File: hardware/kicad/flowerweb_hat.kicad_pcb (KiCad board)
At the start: 2 copper layers, 65 x 56.5 mm, 18 parts, among them J1 PJ-063AH, J2 PJ-063AH, J3 Raspberry Pi 40-pin, J4 STATUS LED, Q1 TIP121, U1 MT3608 module

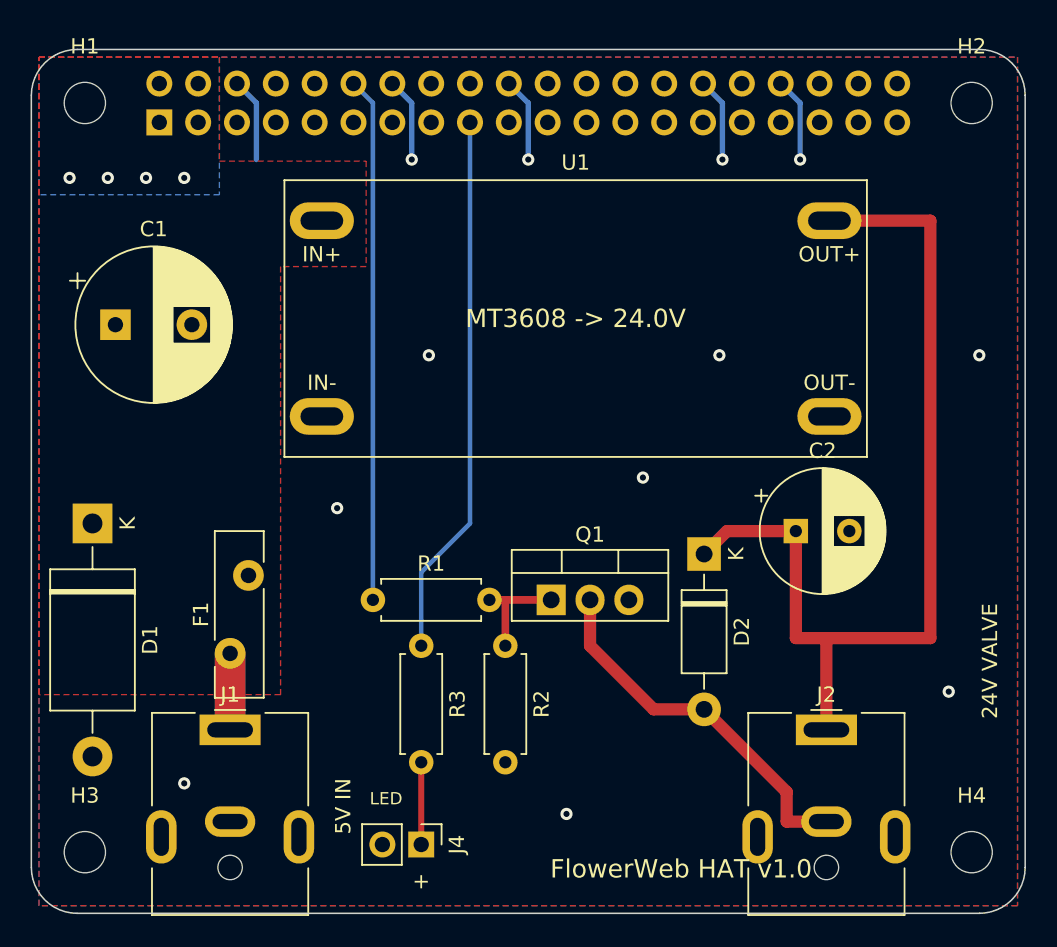
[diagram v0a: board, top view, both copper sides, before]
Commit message: bug fixes
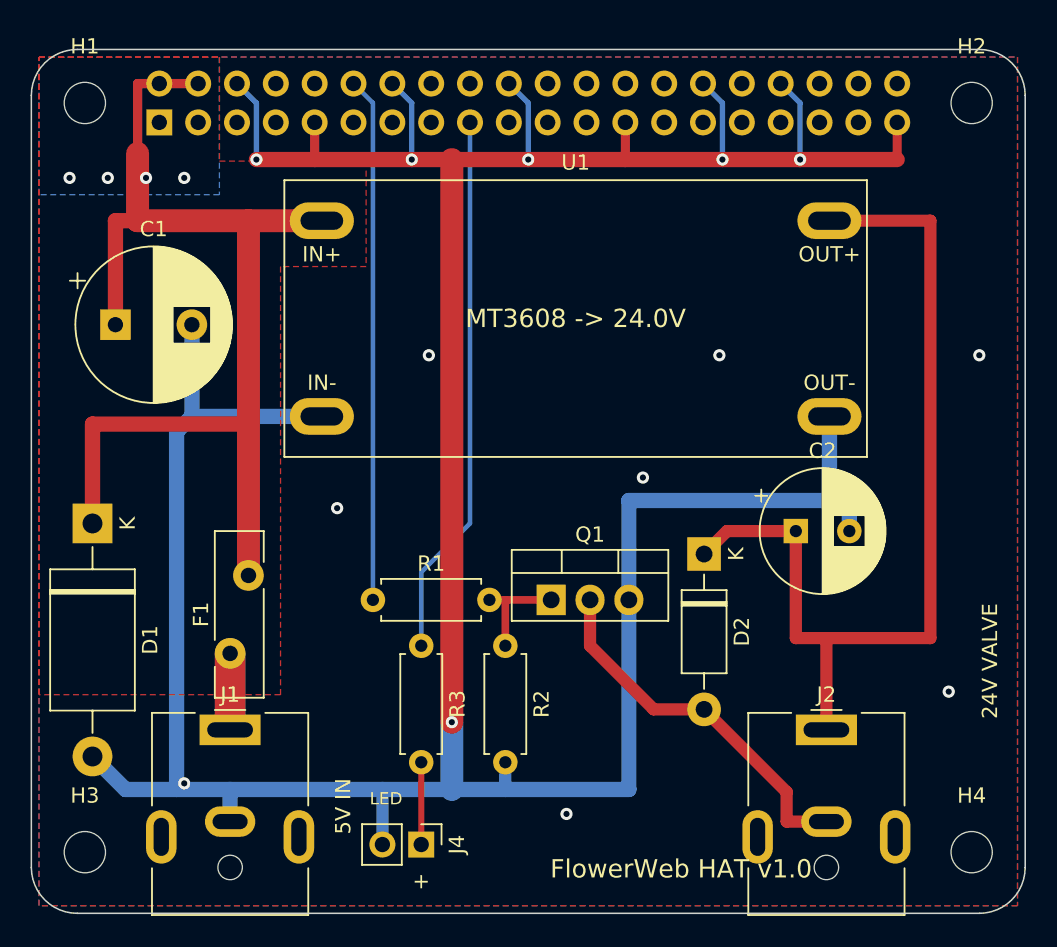
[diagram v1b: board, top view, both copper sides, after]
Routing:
- net GND: track 27.5 -> 241.5 mm, vias 12 -> 14
- net +5V: track 0.00 -> 83.4 mm
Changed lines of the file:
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@@
   (segment (start 149.01 102.23) (end 150.28 103.5) (width 0.35) (layer "B.Cu") (net 1))
   (segment (start 150.28 103.5) (end 150.28 107.2) (width 0.35) (layer "B.Cu") (net 1))
+  (segment (start 114.2 134.4) (end 114.2 111.2) (width 1.5) (layer "F.Cu") (net 2))
+  (segment (start 114.2 111.2) (end 119 111.2) (width 1.5) (layer "F.Cu") (net 2))
+  (segment (start 114.2 111.2) (end 106.95 111.2) (width 1.5) (layer "F.Cu") (net 2))
+  (segment (start 106.95 111.2) (end 106.95 106.8) (width 1.5) (layer "F.Cu") (net 2))
+  (segment (start 106.95 106.8) (end 106.95 102.23) (width 0.6) (layer "F.Cu") (net 2))
+  (segment (start 106.95 102.23) (end 108.37 102.23) (width 0.6) (layer "F.Cu") (net 2))
+  (segment (start 108.37 102.23) (end 110.91 102.23) (width 0.6) (layer "F.Cu") (net 2))
+  (segment (start 107.5 108.4) (end 106.95 106.8) (width 0.6) (layer "B.Cu") (net 2))
+  (segment (start 106.95 106.8) (end 106.95 102.23) (width 0.6) (layer "B.Cu") (net 2))
+  (segment (start 106.95 102.23) (end 108.37 102.23) (width 0.6) (layer "B.Cu") (net 2))
+  (segment (start 108.37 102.23) (end 110.91 102.23) (width 0.6) (layer "B.Cu") (net 2))
+  (segment (start 105.5 118) (end 105.5 111.2) (width 1) (layer "F.Cu") (net 2))
+  (segment (start 105.5 111.2) (end 106.95 111.2) (width 1) (layer "F.Cu") (net 2))
+  (segment (start 104 131) (end 104 124.5) (width 1) (layer "F.Cu") (net 2))
+  (segment (start 104 124.5) (end 114.2 124.5) (width 1) (layer "F.Cu") (net 2))
+  (segment (start 114.72 107.2) (end 118.53 107.2) (width 1) (layer "F.Cu") (net 1))
+  (segment (start 118.53 107.2) (end 124.88 107.2) (width 1) (layer "F.Cu") (net 1))
+  (segment (start 124.88 107.2) (end 127.5 107.2) (width 1) (layer "F.Cu") (net 1))
+  (segment (start 127.5 107.2) (end 132.5 107.2) (width 1) (layer "F.Cu") (net 1))
+  (segment (start 132.5 107.2) (end 138.85 107.2) (width 1) (layer "F.Cu") (net 1))
+  (segment (start 138.85 107.2) (end 145.2 107.2) (width 1) (layer "F.Cu") (net 1))
+  (segment (start 145.2 107.2) (end 150.28 107.2) (width 1) (layer "F.Cu") (net 1))
+  (segment (start 150.28 107.2) (end 156.63 107.2) (width 1) (layer "F.Cu") (net 1))
+  (segment (start 118.53 104.77) (end 118.53 107.2) (width 0.6) (layer "F.Cu") (net 1))
+  (segment (start 138.85 104.77) (end 138.85 107.2) (width 0.6) (layer "F.Cu") (net 1))
+  (segment (start 156.63 104.77) (end 156.63 107.2) (width 0.6) (layer "F.Cu") (net 1))
+  (segment (start 127.5 107.2) (end 127.5 144) (width 1.5) (layer "F.Cu") (net 1))
+  (segment (start 127.5 144) (end 127.5 148.4) (width 1.5) (layer "B.Cu") (net 1))
+  (segment (start 104 146.24) (end 106.16 148.4) (width 1) (layer "B.Cu") (net 1))
+  (segment (start 106.16 148.4) (end 109.5 148.4) (width 1) (layer "B.Cu") (net 1))
+  (segment (start 109.5 148.4) (end 113 148.4) (width 1) (layer "B.Cu") (net 1))
+  (segment (start 113 148.4) (end 122.96 148.4) (width 1) (layer "B.Cu") (net 1))
+  (segment (start 122.96 148.4) (end 127.5 148.4) (width 1) (layer "B.Cu") (net 1))
+  (segment (start 127.5 148.4) (end 131 148.4) (width 1) (layer "B.Cu") (net 1))
+  (segment (start 131 148.4) (end 139.08 148.4) (width 1) (layer "B.Cu") (net 1))
+  (segment (start 113 148.4) (end 113 150.5) (width 1) (layer "B.Cu") (net 1))
+  (segment (start 122.96 148.4) (end 122.96 152) (width 0.8) (layer "B.Cu") (net 1))
+  (segment (start 131 148.4) (end 131 146.62) (width 0.8) (layer "B.Cu") (net 1))
+  (segment (start 109.5 148.4) (end 109.5 125) (width 1) (layer "B.Cu") (net 1))
+  (segment (start 109.5 125) (end 110.5 124) (width 1) (layer "B.Cu") (net 1))
+  (segment (start 110.5 124) (end 119 124) (width 1) (layer "B.Cu") (net 1))
+  (segment (start 110.5 124) (end 110.5 118) (width 1) (layer "B.Cu") (net 1))
+  (segment (start 139.08 148.4) (end 139.08 136) (width 1) (layer "B.Cu") (net 1))
+  (segment (start 139.08 136) (end 139.08 129.5) (width 1) (layer "B.Cu") (net 1))
+  (segment (start 139.08 129.5) (end 152.2 129.5) (width 1) (layer "B.Cu") (net 1))
+  (segment (start 152.2 129.5) (end 153.5 129.5) (width 1) (layer "B.Cu") (net 1))
+  (segment (start 153.5 129.5) (end 153.5 131.5) (width 1) (layer "B.Cu") (net 1))
+  (segment (start 152.2 129.5) (end 152.2 124) (width 1) (layer "B.Cu") (net 1))
+  (via (at 114.72 107.2) (size 0.8) (drill 0.4) (layers "F.Cu" "B.Cu") (net 1))
+  (via (at 127.5 144) (size 0.8) (drill 0.4) (layers "F.Cu" "B.Cu") (net 1))
   (via (at 124.88 107.2) (size 0.8) (drill 0.4) (layers "F.Cu" "B.Cu") (net 1))
   (via (at 132.5 107.2) (size 0.8) (drill 0.4) (layers "F.Cu" "B.Cu") (net 1))
